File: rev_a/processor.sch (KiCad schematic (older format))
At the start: 29 parts, among them J1 TERMINATE_JUMPER, SW1 2_LEAD_PUSH_BUTTON, U1 VOLTAGE_REGULATOR, U2 MCP2562, U3 VOLTAGE_REGULATOR, U4 74x06, U5 ATMEGA324_DIP40, X1 16MHz

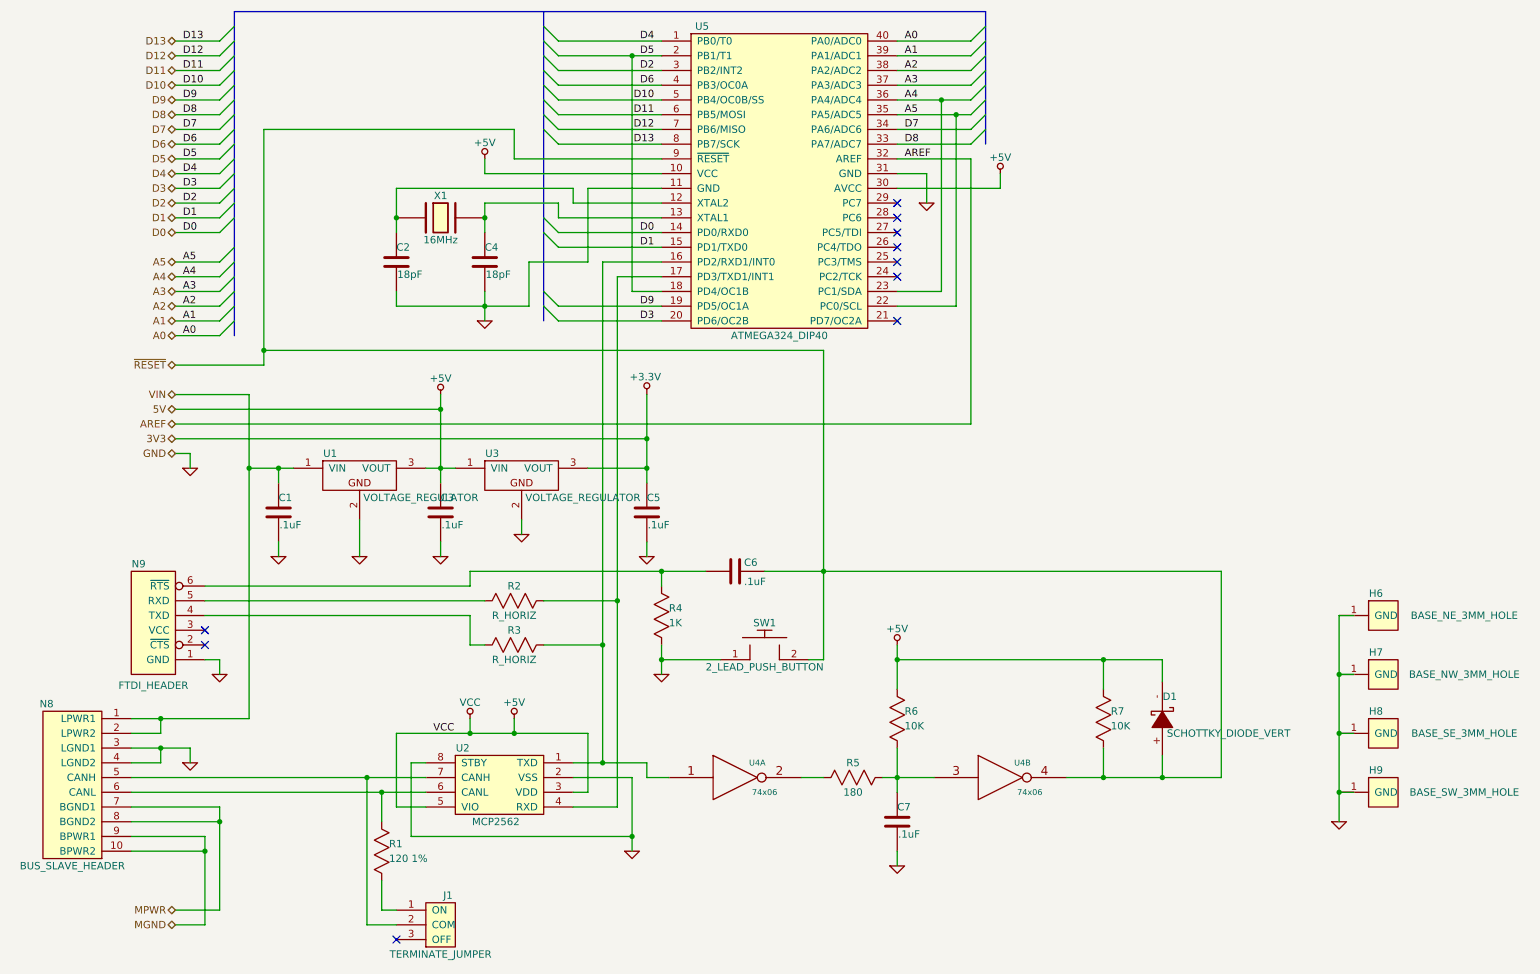
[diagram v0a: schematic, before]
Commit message: Worked on board.
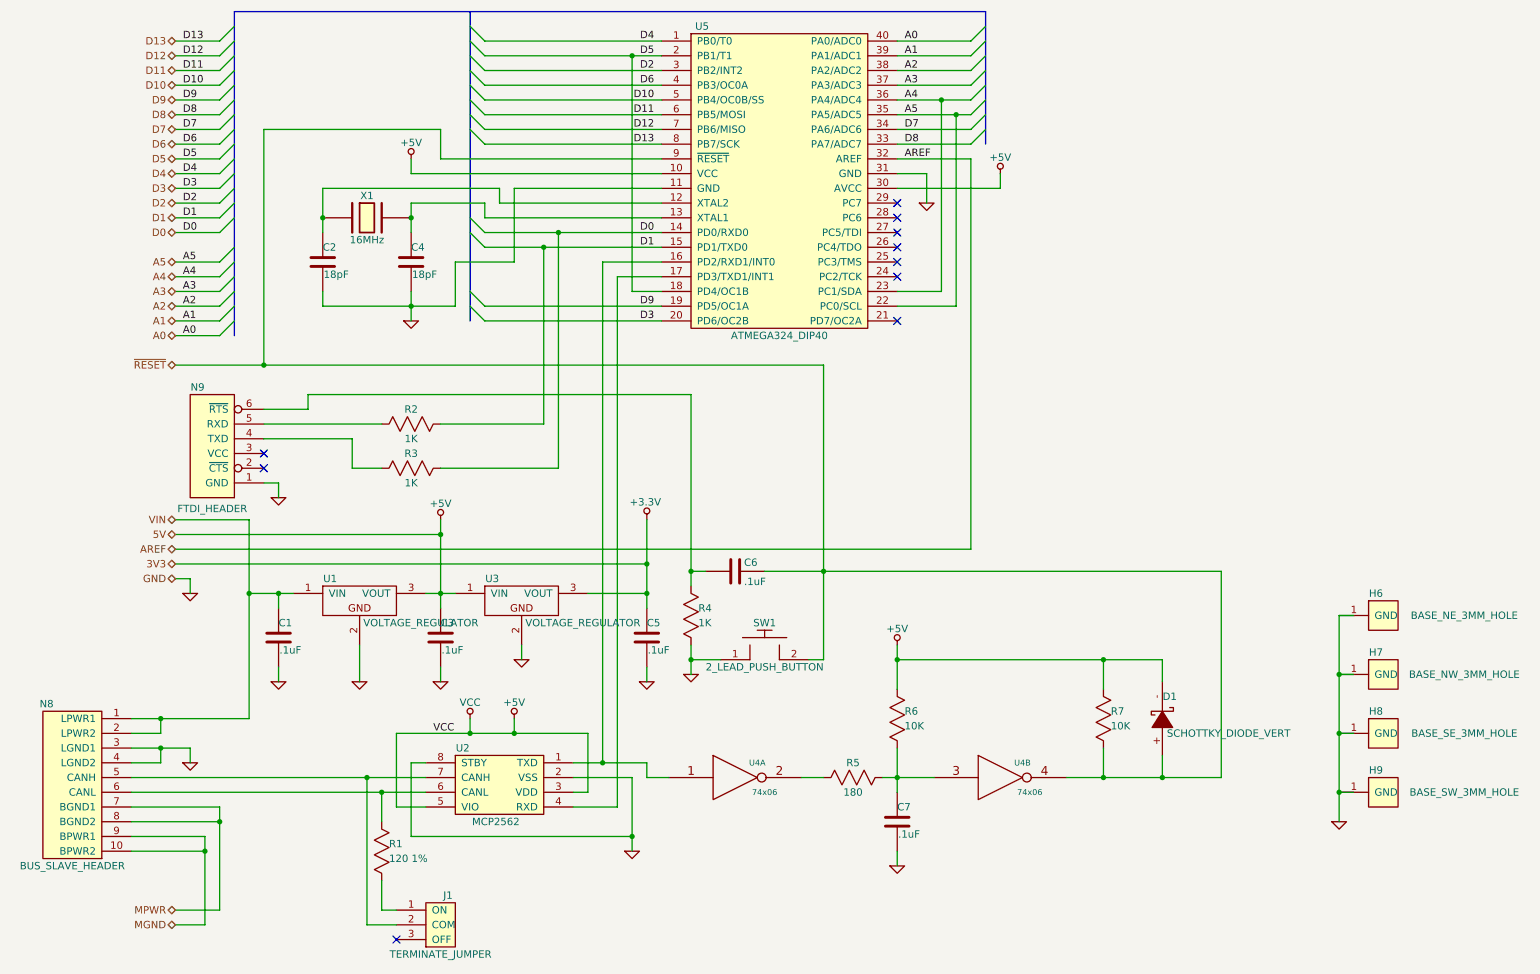
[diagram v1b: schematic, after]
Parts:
- R2, R3: value R_HORIZ -> 1K
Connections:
- net D0: now also R3.2
- net D1: now also R2.2
- net at U2.1 (TXD), U4.1, U5.16 (PD2/RXD1/INT0): no longer R3.2
- net at U2.4 (RXD), U5.17 (PD3/TXD1/INT1): no longer R2.2
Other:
- moved on the sheet: C1, C2, C3, C4, C5, N9, R2, R3, R4, U1, U3, X1
